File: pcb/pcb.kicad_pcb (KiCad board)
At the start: 2 copper layers, 35 parts, among them J1 upd_song, J2 select, J3 swd, SW1 menu, U1 ME2108A, U2 XC6206P333MR, U3 STM32F103C6Tx, U4 TDA2822, U5 AT25xxx

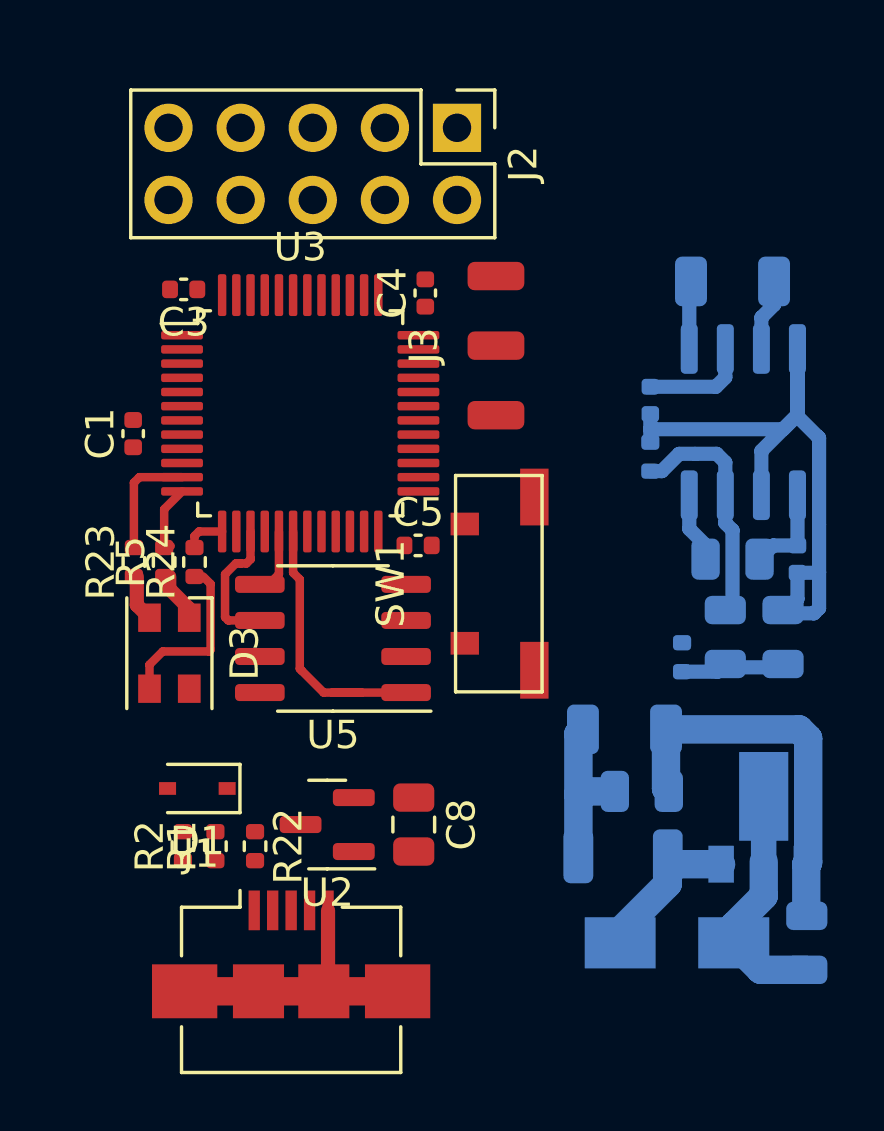
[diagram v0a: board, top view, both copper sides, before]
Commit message: pcb ok
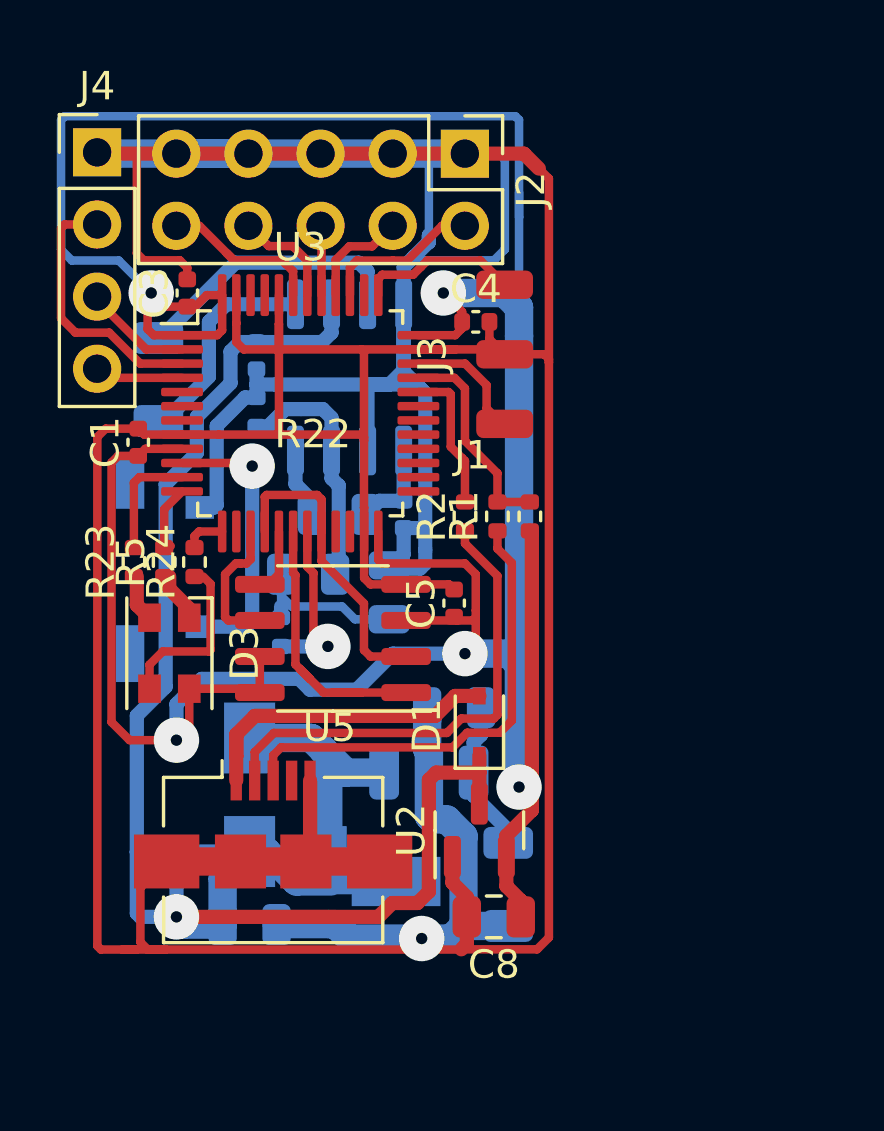
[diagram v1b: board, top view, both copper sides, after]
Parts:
- added J4: buttons, Connector_PinHeader_2.54mm:PinHeader_1x04_P2.54mm_Vertical, F.Cu at (114.7, 53.3)
- SW1: moved to B.Cu
- moved LS1 20.5 mm to (116.8, 61.3), turned to 90 degrees
- moved C7 19.6 mm to (120.1, 80.5), turned to 0 degrees
- moved D2 15.9 mm to (120.1, 76.0), turned to 90 degrees
- moved R1 15.3 mm to (128.8, 66.2)
- moved R2 15.3 mm to (127.6, 66.2)
- moved R22 15.1 mm to (129.9, 66.2), turned to 90 degrees
- moved C10 14.9 mm to (122.1, 68.2), turned to 0 degrees
- moved R3 14.2 mm to (121.2, 70.2), turned to 90 degrees
- moved C6 14.0 mm to (120.3, 60.5)
- moved C11 14.0 mm to (123.2, 66.1)
- moved C12 14.0 mm to (125.5, 66.1)
- moved R4 14.0 mm to (120.3, 62.5)
- moved U4 14.0 mm to (123.6, 61.3)
- moved C9 14.0 mm to (125.0, 68.8)
- moved U1 13.9 mm to (124.5, 79.0), turned to 0 degrees
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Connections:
- R22 pad 1: +5V -> +3.3V
- U3 pad 10: unconnected-(U3-Pad10) -> Net-(SW1-Pad2)
- U3 pad 16: Net-(U3-Pad16) -> Net-(U3-Pad20)
- U3 pad 2: unconnected-(U3-Pad2) -> Net-(J4-Pad3)
- U3 pad 20: unconnected-(U3-Pad20) -> Net-(U3-Pad20)
- U3 pad 3: unconnected-(U3-Pad3) -> Net-(U3-Pad3)
- U3 pad 4: unconnected-(U3-Pad4) -> Net-(J4-Pad4)
- U3 pad 46: Net-(SW1-Pad2) -> unconnected-(U3-Pad46)
- U5 pad 2: Net-(U3-Pad16) -> Net-(U3-Pad20)
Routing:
- net GND: track 49.3 -> 239.0 mm, vias 0 -> 1
- net +3.3V: track 0.00 -> 128.0 mm, vias 0 -> 5
- net +5V: track 10.9 -> 60.5 mm, vias 0 -> 1
- net Net-(J1-Pad2): track 0.00 -> 17.0 mm
- net Net-(J1-Pad3): track 0.00 -> 16.7 mm
- net Net-(D1-Pad2): track 0.00 -> 11.4 mm
- net Net-(U3-Pad20): track 0.00 -> 10.8 mm
- net Net-(SW1-Pad2): track 0.00 -> 9.45 mm, vias 0 -> 1
- net Net-(U3-Pad3): track 0.00 -> 9.42 mm
- net Net-(LS1-Pad2): track 2.56 -> 10.8 mm
- net Net-(R22-Pad2): track 0.00 -> 7.41 mm
- net Net-(J2-Pad10): track 0.00 -> 6.12 mm
- net Net-(LS1-Pad1): track 2.40 -> 8.44 mm
- net Net-(J3-Pad3): track 0.00 -> 6.02 mm
- net Net-(R3-Pad1): track 0.00 -> 6.00 mm, vias 0 -> 1
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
